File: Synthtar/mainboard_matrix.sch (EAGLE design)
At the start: 79 parts, among them IC1 74HC164N, IC2 4081N, IC3 555, IC4 4081N, J1 AUDIO_JACK_3.5MM_PTH, M1 ARDUINO-NANO-3.0, X1 HD44780LCD-1602, X2 MINI-USB-UX60A-MB-5ST

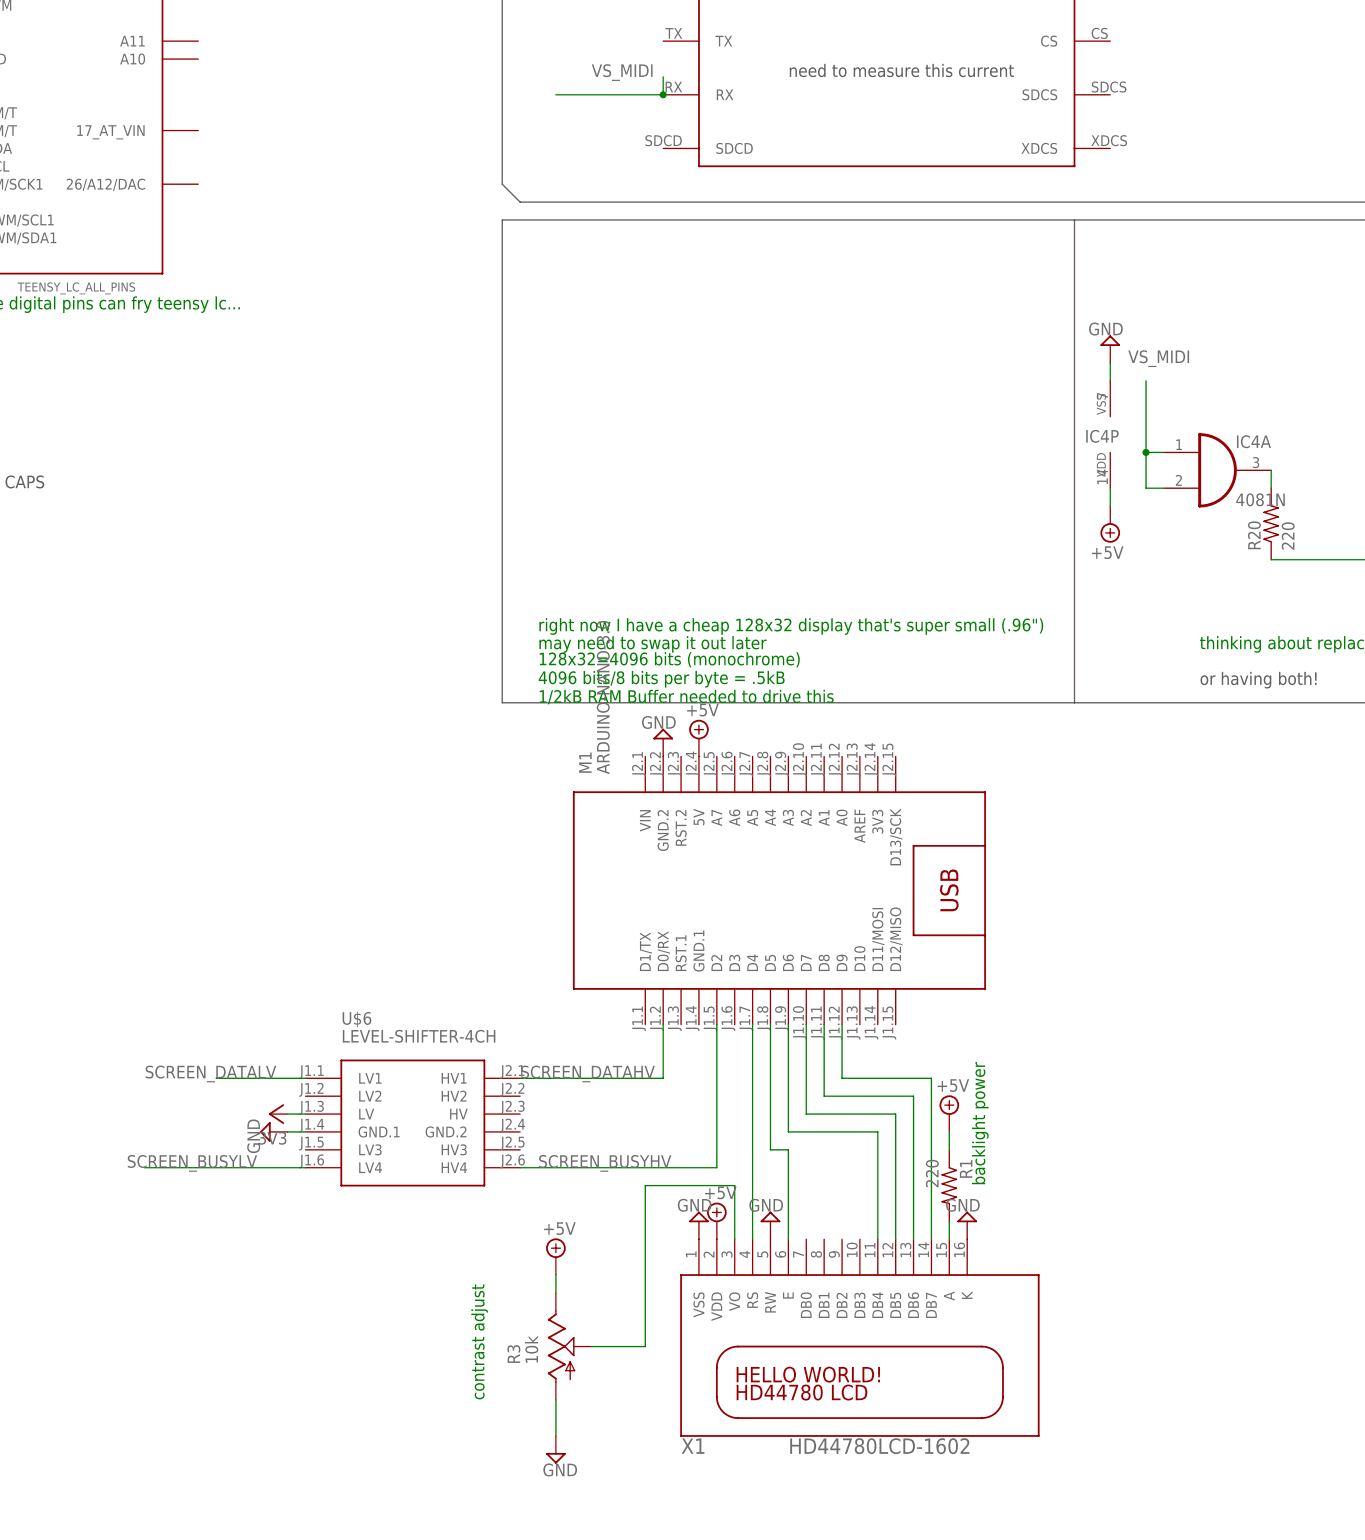
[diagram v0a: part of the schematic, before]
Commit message: more uploads
more recent files. code improvements
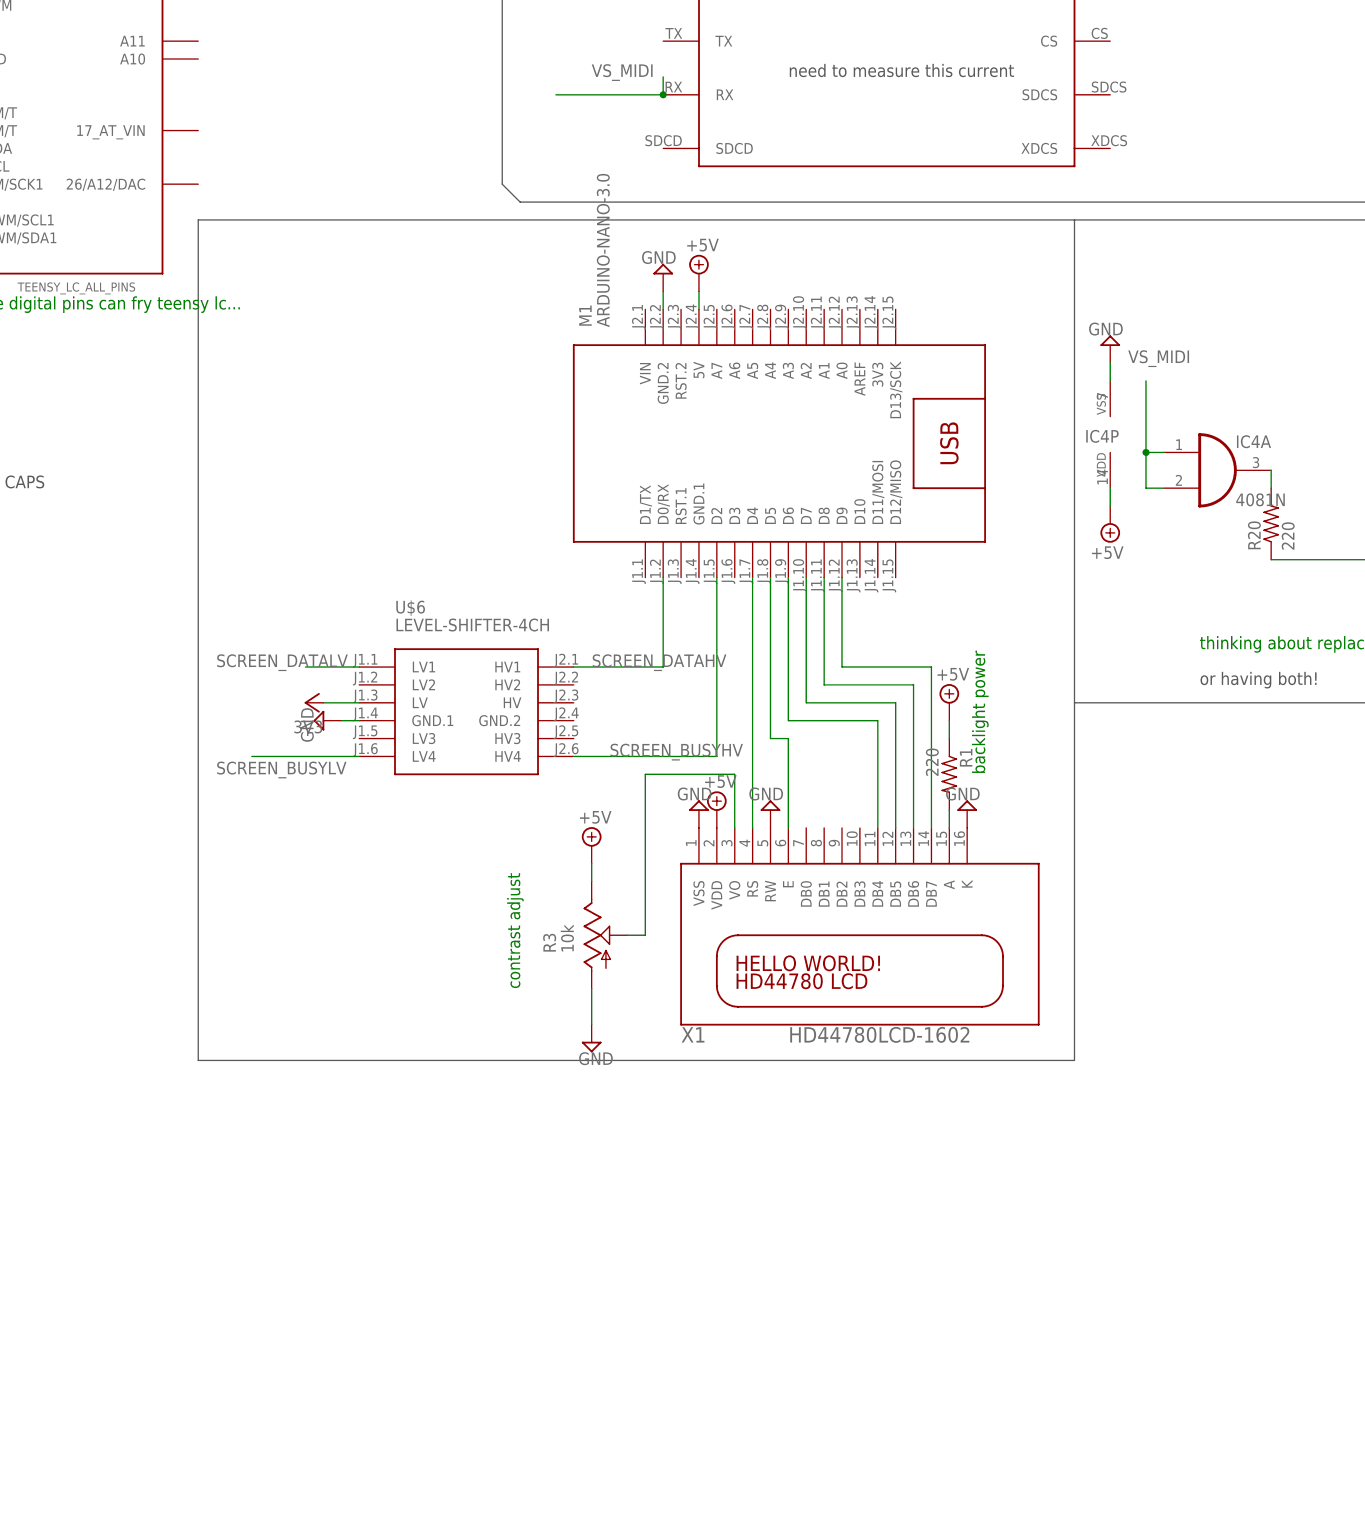
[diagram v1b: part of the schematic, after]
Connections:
- net GND: now also M1.GND.2, X1.RW
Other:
- note removed: "128x32=4096 bits (monochrome) 4096 bits/8 bits per byte = .5kB 1/2kB RAM Buffer needed to drive this"
- note removed: "may need to swap it out later"
- note removed: "right now I have a cheap 128x32 display that's super small (.96")"
- moved on the sheet: M1, R1, R3, U$6, X1
